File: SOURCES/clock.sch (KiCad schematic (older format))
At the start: 6 parts, among them U10 IDT2309NZ, X1 Crystal_Oszillator

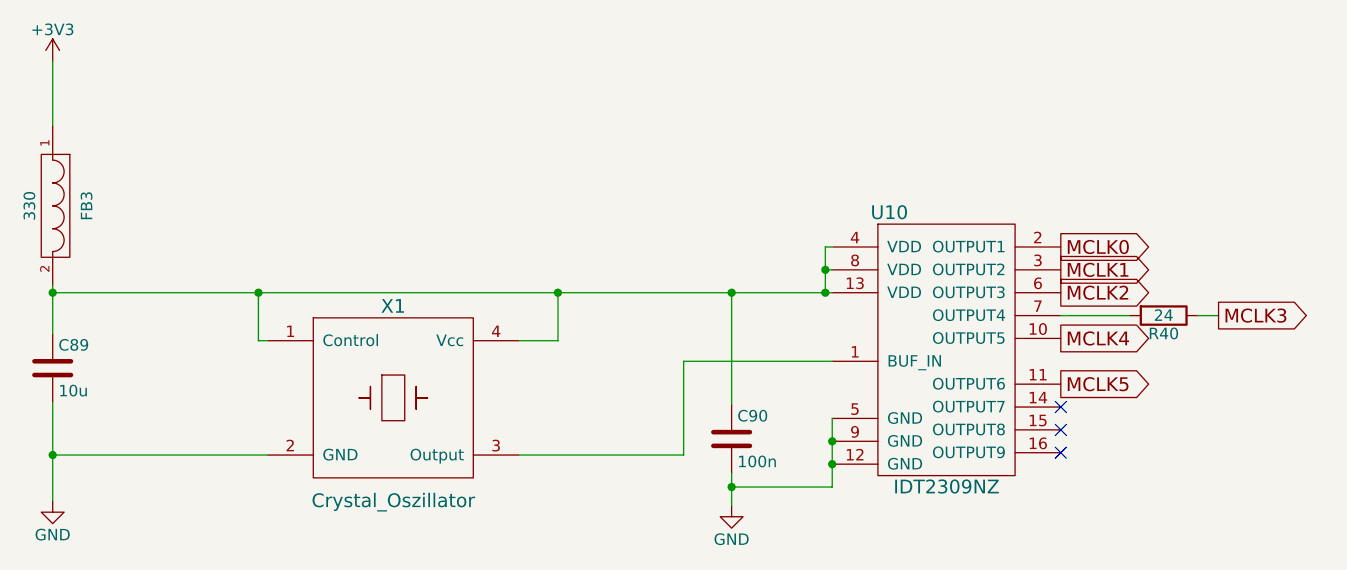
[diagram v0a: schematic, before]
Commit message: finished drc
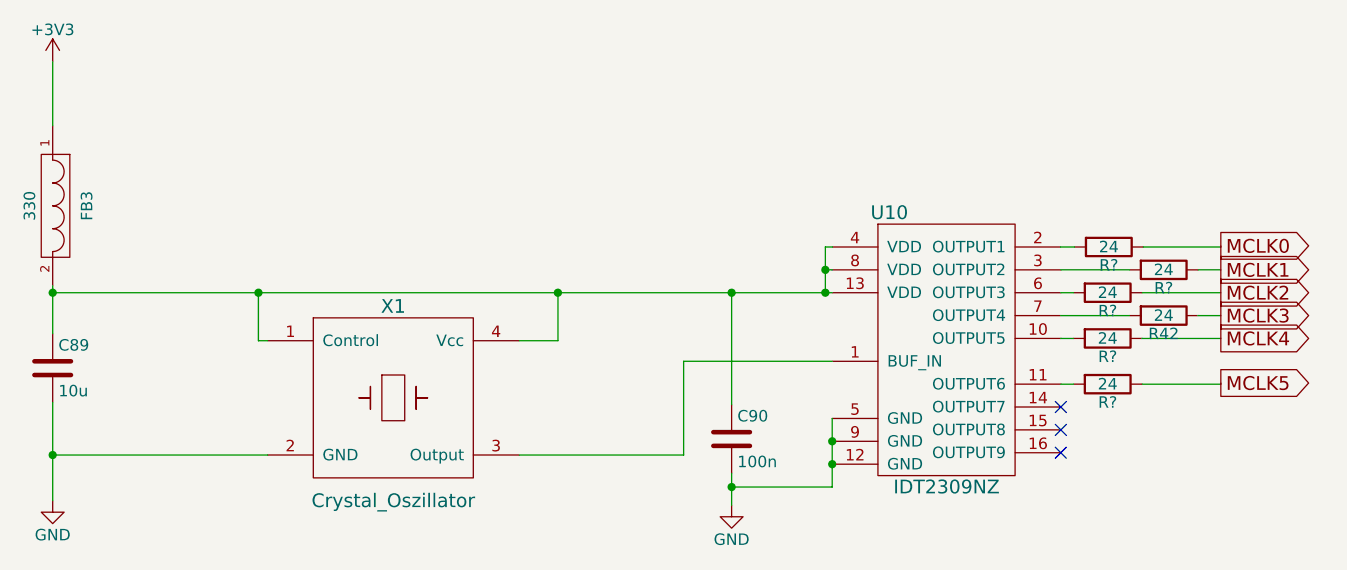
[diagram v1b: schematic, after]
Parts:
- added R? (x5): 24, symbol R
- renumbered R40 to R42
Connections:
- net MCLK0: now also R?.1; no longer U10.2 (OUTPUT1)
- net MCLK1: now also R?.1; no longer U10.3 (OUTPUT2)
- net MCLK2: now also R?.1; no longer U10.6 (OUTPUT3)
- net MCLK4: now also R?.1; no longer U10.10 (OUTPUT5)
- net MCLK5: now also R?.1; no longer U10.11 (OUTPUT6)
- new net: R?.2, U10.10 (OUTPUT5)
- new net: R?.2, U10.11 (OUTPUT6)
- new net: R?.2, U10.2 (OUTPUT1)
- new net: R?.2, U10.3 (OUTPUT2)
- new net: R?.2, U10.6 (OUTPUT3)
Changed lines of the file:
@@
 $EndComp
 $Comp
-L +3V3 #PWR0131
+L +3V3 #PWR0139
 U 1 1 5B071680
 P 3050 1930
-F 0 "#PWR0131" H 3050 1780 50  0001 C CNN
+F 0 "#PWR0139" H 3050 1780 50  0001 C CNN
 F 1 "+3V3" H 3050 2070 50  0000 C CNN
 F 2 "" H 3050 1930 60  0000 C CNN
@@
 $EndComp
 $Comp
-L GND #PWR0132
+L GND #PWR0140
 U 1 1 5B071722
 P 3050 3850
-F 0 "#PWR0132" H 3050 3600 50  0001 C CNN
+F 0 "#PWR0140" H 3050 3600 50  0001 C CNN
 F 1 "GND" H 3050 3700 50  0000 C CNN
 F 2 "" H 3050 3850 60  0000 C CNN
@@
 	1    0    0    -1
 $EndComp
-Text GLabel 7460 2740 2    60   Output ~ 0
+Text GLabel 8160 2735 2    60   Output ~ 0
 MCLK0
-Text GLabel 7460 2840 2    60   Output ~ 0
+Text GLabel 8160 2840 2    60   Output ~ 0
 MCLK1
-Text GLabel 8150 3040 2    60   Output ~ 0
+Text GLabel 8160 3040 2    60   Output ~ 0
 MCLK3
-Text GLabel 7460 2940 2    60   Output ~ 0
+Text GLabel 8160 2940 2    60   Output ~ 0
 MCLK2
-Text GLabel 7460 3340 2    60   Output ~ 0
+Text GLabel 8160 3335 2    60   Output ~ 0
 MCLK5
 $Comp
@@
 $EndComp
 $Comp
-L GND #PWR0133
+L GND #PWR0141
 U 1 1 5B0732C4
 P 6020 3870
-F 0 "#PWR0133" H 6020 3620 50  0001 C CNN
+F 0 "#PWR0141" H 6020 3620 50  0001 C CNN
 F 1 "GND" H 6020 3720 50  0000 C CNN
 F 2 "" H 6020 3870 60  0000 C CNN
@@
 	1    0    0    -1
 $EndComp
-Text GLabel 7460 3140 2    60   Output ~ 0
+Text GLabel 8160 3140 2    60   Output ~ 0
 MCLK4
 $Comp
@@
 Connection ~ 3050 2940
 Wire Wire Line
-	3050 3420 3050 3850
-Wire Wire Line
-	3050 2910 3050 3120
+	3050 3420 3050 3650
+Wire Wire Line
+	3050 3650 3050 3850
+Wire Wire Line
+	3050 2910 3050 2940
+Wire Wire Line
+	3050 2940 3050 3120
 Wire Wire Line
 	3050 1930 3050 2210
@@
 	5810 3240 6460 3240
 Wire Wire Line
-	6020 3870 6020 3730
+	6020 3730 6020 3790
+Wire Wire Line
+	6020 3790 6020 3870
 Wire Wire Line
 	6460 3790 6020 3790
 Wire Wire Line
-	6460 3490 6460 3790
+	6460 3490 6460 3590
+Wire Wire Line
+	6460 3590 6460 3690
+Wire Wire Line
+	6460 3690 6460 3790
 Connection ~ 6020 3790
 Connection ~ 6460 3690
 Connection ~ 6460 3590
 Wire Wire Line
-	3050 2940 6460 2940
-Wire Wire Line
-	6430 2740 6430 2940
+	3050 2940 3950 2940
+Wire Wire Line
+	3950 2940 5260 2940
+Wire Wire Line
+	5260 2940 6020 2940
+Wire Wire Line
+	6020 2940 6430 2940
+Wire Wire Line
+	6430 2940 6460 2940
+Wire Wire Line
+	6430 2740 6430 2840
+Wire Wire Line
+	6430 2840 6430 2940
 Wire Wire Line
 	6430 2840 6460 2840
@@
 Connection ~ 6020 2940
 $Comp
-L R R40
+L R R42
 U 1 1 5B1890A3
 P 7910 3040
-F 0 "R40" V 7990 3040 50  0000 C CNN
+F 0 "R42" V 7990 3040 50  0000 C CNN
 F 1 "24" V 7910 3040 50  0000 C CNN
 F 2 "" V 7840 3040 30  0000 C CNN
@@
 	7460 3040 7760 3040
 Wire Wire Line
-	8060 3040 8150 3040
+	8060 3040 8160 3040
+$Comp
+L R R?
+U 1 1 5B1F732A
+P 7665 2940
+F 0 "R?" V 7745 2940 50  0000 C CNN
+F 1 "24" V 7665 2940 50  0000 C CNN
+F 2 "" V 7595 2940 30  0000 C CNN
+F 3 "" H 7665 2940 30  0000 C CNN
+	1    7665 2940
+	0    1    1    0
+$EndComp
+Wire Wire Line
+	7460 2940 7515 2940
+Wire Wire Line
+	7815 2940 8160 2940
+$Comp
+L R R?
+U 1 1 5B1F742C
+P 7910 2840
+F 0 "R?" V 7990 2840 50  0000 C CNN
+F 1 "24" V 7910 2840 50  0000 C CNN
+F 2 "" V 7840 2840 30  0000 C CNN
+F 3 "" H 7910 2840 30  0000 C CNN
+	1    7910 2840
+	0    1    1    0
+$EndComp
+$Comp
+L R R?
+U 1 1 5B1F7478
+P 7670 2740
+F 0 "R?" V 7750 2740 50  0000 C CNN
+F 1 "24" V 7670 2740 50  0000 C CNN
+F 2 "" V 7600 2740 30  0000 C CNN
+F 3 "" H 7670 2740 30  0000 C CNN
+	1    7670 2740
+	0    1    1    0
+$EndComp
+Wire Wire Line
+	7460 2740 7520 2740
+Wire Wire Line
+	7820 2740 8160 2740
+Wire Wire Line
+	8160 2740 8160 2735
+Wire Wire Line
+	7460 2840 7760 2840
+Wire Wire Line
+	8060 2840 8160 2840
+$Comp
+L R R?
+U 1 1 5B1F76D9
+P 7665 3140
+F 0 "R?" V 7745 3140 50  0000 C CNN
+F 1 "24" V 7665 3140 50  0000 C CNN
+F 2 "" V 7595 3140 30  0000 C CNN
+F 3 "" H 7665 3140 30  0000 C CNN
+	1    7665 3140
+	0    1    1    0
+$EndComp
+Wire Wire Line
+	7460 3140 7515 3140
+Wire Wire Line
+	7815 3140 8160 3140
+$Comp
+L R R?
+U 1 1 5B1F7927
+P 7665 3340
+F 0 "R?" V 7745 3340 50  0000 C CNN
+F 1 "24" V 7665 3340 50  0000 C CNN
+F 2 "" V 7595 3340 30  0000 C CNN
+F 3 "" H 7665 3340 30  0000 C CNN
+	1    7665 3340
+	0    1    1    0
+$EndComp
+Wire Wire Line
+	7460 3340 7515 3340
+Wire Wire Line
+	7815 3340 8160 3340
+Wire Wire Line
+	8160 3340 8160 3335
 $EndSCHEMATC
